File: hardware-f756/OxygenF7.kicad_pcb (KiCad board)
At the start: 2 copper layers, 78 x 37 mm, 52 parts, among them J1 Conn_01x04, J10 Micro_SD_Card_Det, J2 USB_C_2.0, J3 JST SH-4, J4 JST ZH-4, J5 Conn_03x08, J6 Conn_01x16, J7 Conn_01x04, J9 1.25mm, SW1 SW_Push, SW2 SW_Push, U1 STM32F756VGTx, U2 XC6220B331MR, U3 MPU-6000, U4 BMP388, Y1 8Mhz

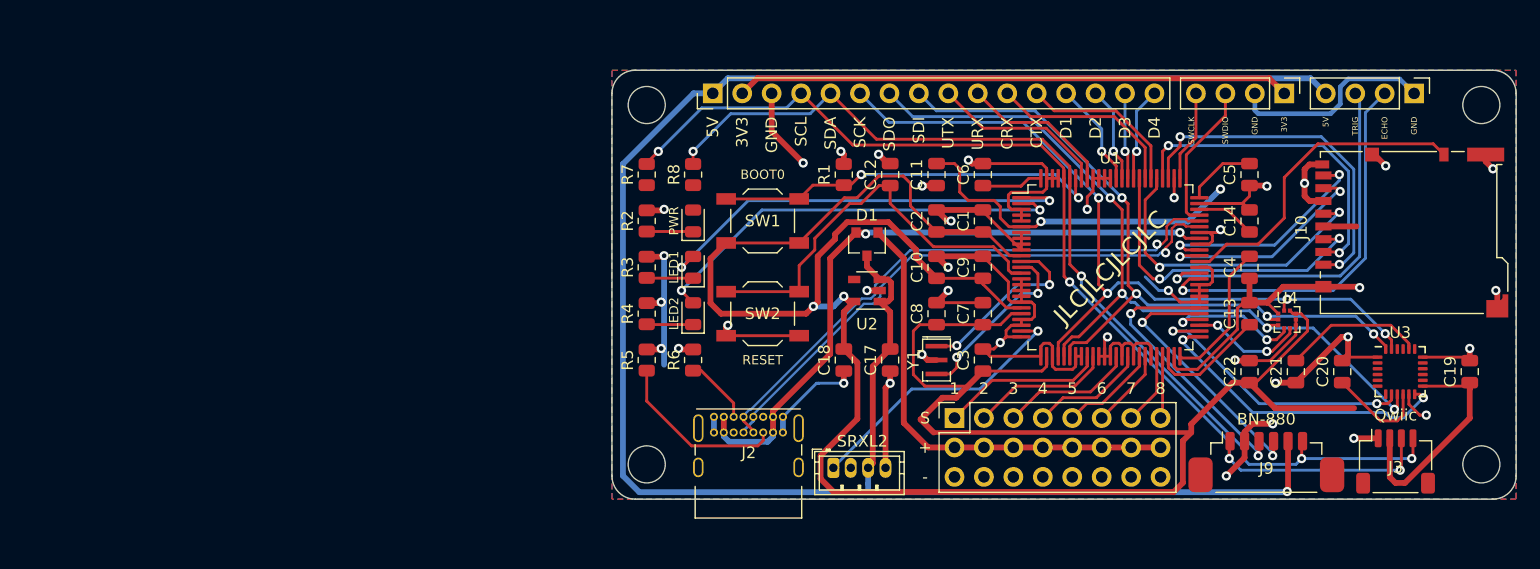
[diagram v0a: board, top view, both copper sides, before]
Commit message: New board layout
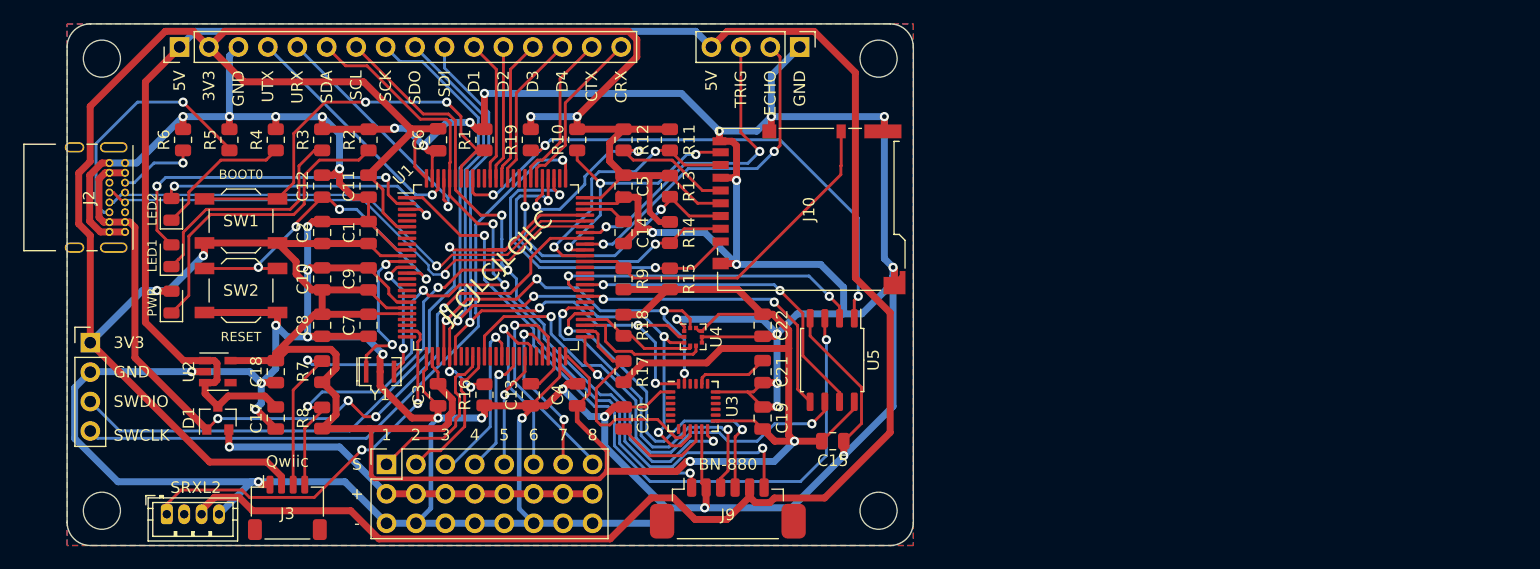
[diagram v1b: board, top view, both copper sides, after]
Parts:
- added C15: 0.1u, Capacitor_SMD:C_0805_2012Metric, F.Cu at (180.1, 114.0)
- added R10: 47k, Resistor_SMD:R_0805_2012Metric, F.Cu at (158.0, 88.0)
- added R11: 47k, Resistor_SMD:R_0805_2012Metric, F.Cu at (166.0, 88.0)
- added R12: 47k, Resistor_SMD:R_0805_2012Metric, F.Cu at (162.0, 88.0)
- added R13: 47k, Resistor_SMD:R_0805_2012Metric, F.Cu at (166.0, 92.0)
- added R14: 47k, Resistor_SMD:R_0805_2012Metric, F.Cu at (166.0, 96.0)
- added R15: 47k, Resistor_SMD:R_0805_2012Metric, F.Cu at (166.0, 100.0)
- added R16: 100k, Resistor_SMD:R_0805_2012Metric, F.Cu at (150.0, 110.0)
- added R17: 10k, Resistor_SMD:R_0805_2012Metric, F.Cu at (162.0, 108.0)
- added R18: 10k, Resistor_SMD:R_0805_2012Metric, F.Cu at (162.0, 104.0)
- added R19: 10k, Resistor_SMD:R_0805_2012Metric, F.Cu at (154.0, 88.0)
- added R9: 10k, Resistor_SMD:R_0805_2012Metric, F.Cu at (162.0, 100.0)
- added U5: W25Q128JVS, Package_SO:SOIC-8_5.23x5.23mm_P1.27mm, F.Cu at (180.0, 107.0)
- moved J1 105.2 mm to (116.0, 105.5), turned to 0 degrees
- moved J3 95.7 mm to (133.0, 119.8)
- moved C13 62.4 mm to (154.0, 110.0), turned to 90 degrees
- moved C20 62.1 mm to (162.0, 112.0)
- moved C19 61.1 mm to (174.0, 112.0)
- moved U3 61.1 mm to (168.0, 111.0)
- moved C4 59.0 mm to (158.0, 110.0), turned to 90 degrees
- moved D1 58.0 mm to (127.0, 112.0), turned to 90 degrees
- moved J4 57.6 mm to (122.6, 120.3)
- moved U2 56.4 mm to (127.0, 108.0), turned to 0 degrees
- moved J2 55.3 mm to (119.0, 90.0), turned to 270 degrees
- moved C14 54.0 mm to (162.0, 96.0), turned to 270 degrees
- moved C5 54.0 mm to (162.0, 92.0)
- moved C17 53.2 mm to (132.0, 112.0)
- moved J7 53.2 mm to (177.2, 80.0)
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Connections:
- D1 pad 1: +5V_BEC -> VBUS
- D1 pad 2: VBUS -> +5V_BEC
- J6 pad 10: USART1_TX -> SPI1_MOSI
- J6 pad 11: CAN1_TX -> GPIO_1
- J6 pad 12: CAN1_RX -> GPIO_2
- J6 pad 13: GPIO_1 -> GPIO_3
- J6 pad 14: GPIO_2 -> GPIO_4
- J6 pad 15: GPIO_3 -> CAN1_TX
- J6 pad 16: GPIO_4 -> CAN1_RX
- J6 pad 4: I2C1_SDA -> UART8_TX
- J6 pad 5: I2C1_SCL -> UART8_RX
- J6 pad 6: SPI1_SCLK -> I2C1_SDA
- J6 pad 7: SPI1_MISO -> I2C1_SCL
- J6 pad 8: SPI1_MOSI -> SPI1_SCLK
- J6 pad 9: USART1_RX -> SPI1_MISO
- U1 pad 1: LED1 -> QUADSPI_IO2
- U1 pad 15: GND -> (no net)
- U1 pad 16: GND -> (no net)
- U1 pad 17: GND -> (no net)
- U1 pad 18: GND -> (no net)
- U1 pad 2: LED2 -> LED1
- U1 pad 22: GND -> (no net)
- U1 pad 23: GND -> (no net)
- U1 pad 25: GND -> (no net)
- U1 pad 28: GND -> (no net)
- U1 pad 3: GND -> LED2
- U1 pad 32: GND -> (no net)
- U1 pad 33: GND -> (no net)
- U1 pad 36: GND -> QUADSPI_SCLK
- U1 pad 37: GND -> (no net)
- U1 pad 38: GND -> (no net)
- U1 pad 4: GND -> (no net)
- U1 pad 40: GND -> (no net)
- U1 pad 42: GND -> (no net)
- U1 pad 45: GND -> (no net)
- U1 pad 5: GND -> (no net)
- U1 pad 57: GND -> (no net)
- U1 pad 58: GND -> QUADSPI_IO0
- U1 pad 59: GND -> QUADSPI_IO1
- U1 pad 60: GND -> QUADSPI_IO3
- U1 pad 61: ULTRA_ECHO -> (no net)
- U1 pad 62: ULTRA_TRIG -> (no net)
- U1 pad 63: GND -> (no net)
- U1 pad 67: GND -> ULTRA_ECHO
- U1 pad 69: GND -> ULTRA_TRIG
- U1 pad 7: GND -> (no net)
- U1 pad 77: GND -> (no net)
- U1 pad 8: GND -> (no net)
- U1 pad 84: GPIO_4 -> (no net)
- U1 pad 85: GPIO_3 -> (no net)
- U1 pad 86: GPIO_2 -> GPIO_4
- U1 pad 87: GPIO_1 -> GPIO_3
- U1 pad 88: GND -> GPIO_2
- U1 pad 89: GND -> GPIO_1
- U1 pad 9: GND -> (no net)
- U1 pad 90: GND -> (no net)
- U1 pad 91: GND -> (no net)
- U1 pad 92: USART1_TX -> QUADSPI_CS
- U1 pad 93: USART1_RX -> (no net)
- U1 pad 97: GND -> UART8_RX
- U1 pad 98: GND -> UART8_TX
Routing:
- net GND: track 259.8 -> 512.7 mm, vias 38 -> 36
- net QUADSPI_IO2: track 0.00 -> 63.9 mm, vias 0 -> 2
- net +3V3: track 342.4 -> 401.1 mm, vias 4 -> 6
- net SWCLK: track 7.90 -> 58.1 mm, vias 0 -> 1
- net QUADSPI_CS: track 0.00 -> 49.5 mm, vias 0 -> 3
- net SWDIO: track 12.9 -> 57.7 mm, vias 0 -> 1
- net QUADSPI_SCLK: track 0.00 -> 42.3 mm, vias 0 -> 2
- net QUADSPI_IO3: track 0.00 -> 28.8 mm, vias 0 -> 2
- net +5V: track 177.1 -> 205.5 mm, vias 1 -> 0
- net QUADSPI_IO1: track 0.00 -> 27.8 mm, vias 0 -> 2
- net QUADSPI_IO0: track 0.00 -> 26.4 mm, vias 0 -> 2
- net Net-(D2-Pad1): track 4.01 -> 27.3 mm
- net UART8_RX: track 0.00 -> 21.8 mm, vias 0 -> 1
- net UART8_TX: track 0.00 -> 21.1 mm, vias 0 -> 1
- net Net-(D3-Pad1): track 4.01 -> 20.0 mm
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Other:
- board size 78 x 37 mm -> 73 x 45 mm
- board text added: "Rev A @ 2021-05"
- board text removed: "Rev A @ 2021-04"
